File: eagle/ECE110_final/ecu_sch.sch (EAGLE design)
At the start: 1 part, among them IC1 MEGA8-AI

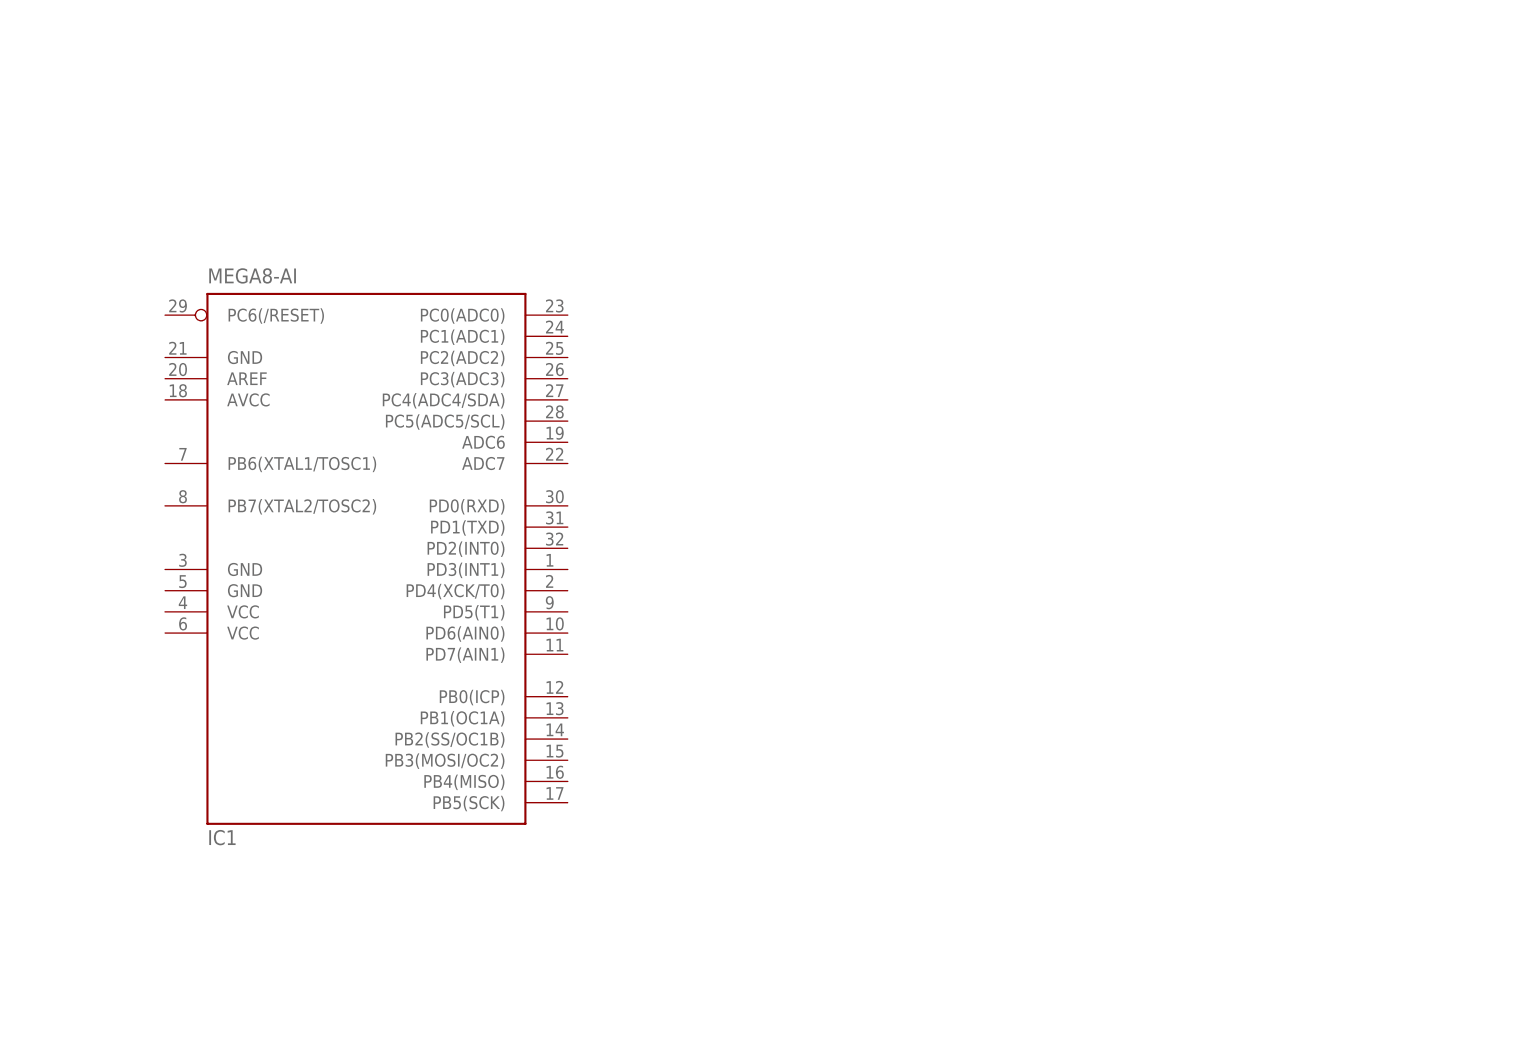
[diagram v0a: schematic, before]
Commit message: ECU Schematics: v1
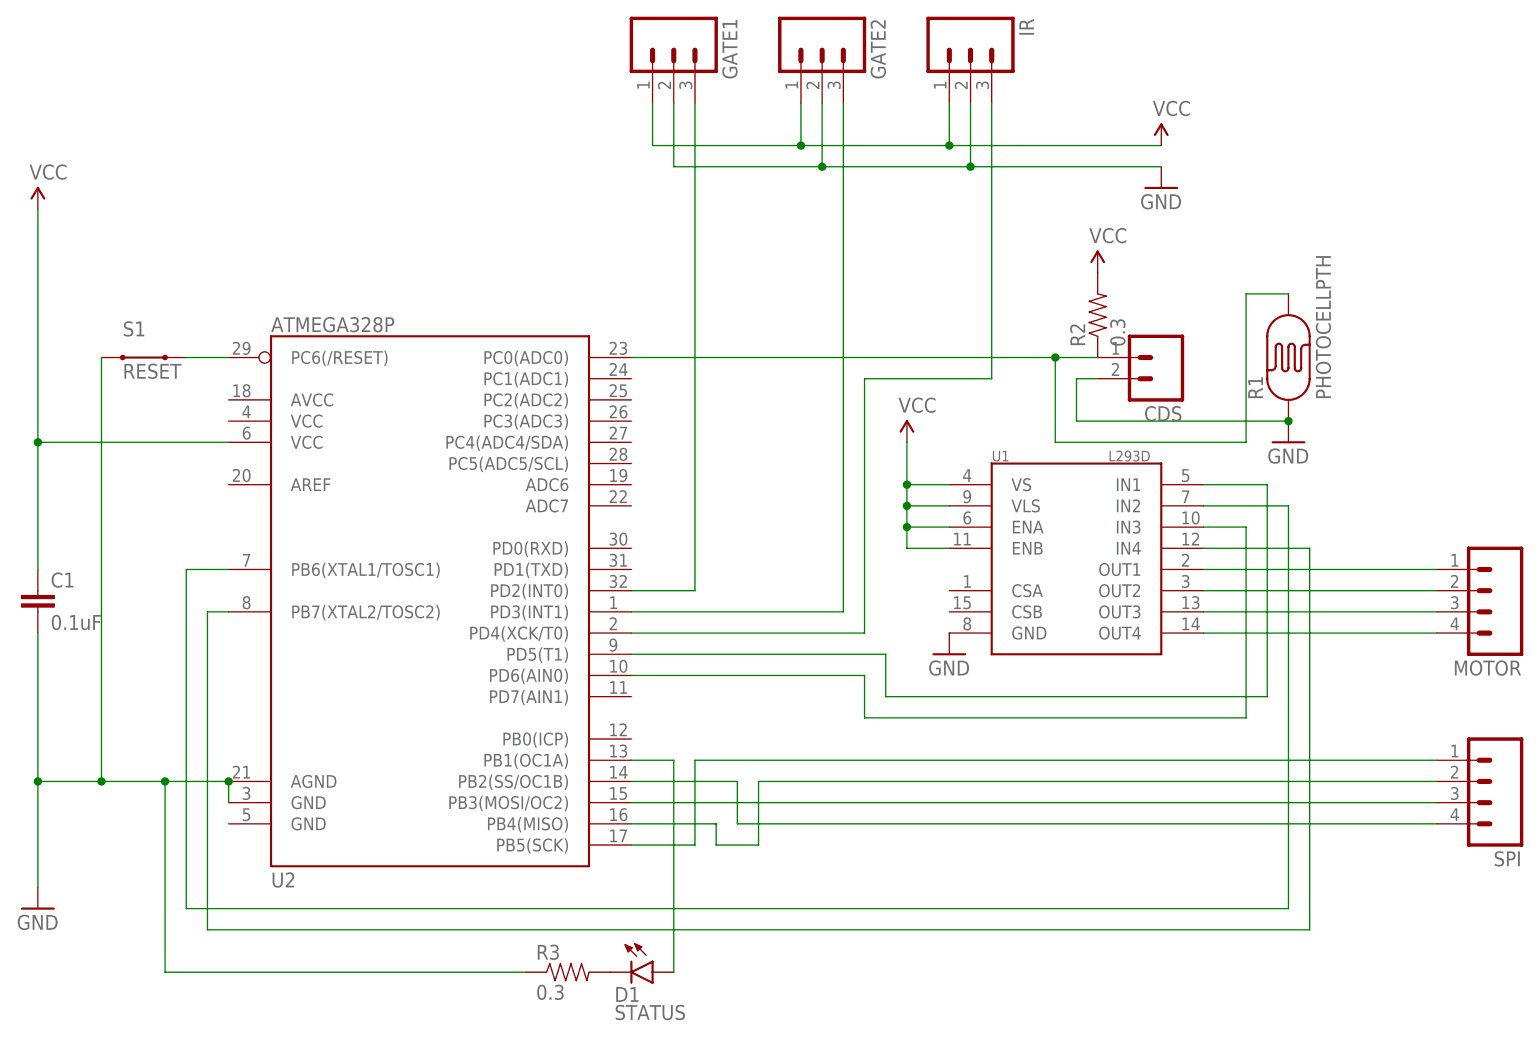
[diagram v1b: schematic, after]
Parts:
- removed IC1: MEGA8-AI, atmel:MEGA8-AI
- added C1: 0.1uF, SparkFun-Capacitors:0.1UF-25V(+80/-20%)(0603)
- added CDS: M02JST-PTH-2, SparkFun-Connectors:M02JST-PTH-2
- added D1: STATUS, SparkFun-LED:LED-WHITE
- added GATE1, GATE2, IR: (no value), SparkFun-Connectors:M03JST-PTH
- added MOTOR, SPI: (no value), SparkFun-Connectors:M04JST-PTH
- added R1: PHOTOCELLPTH, SparkFun-Sensors:PHOTOCELLPTH
- added R2, R3: 0.3, SparkFun-Resistors:0.3OHM-1/8W-1%(0805)
- added S1: RESET, SparkFun-Electromechanical:SWITCH-MOMENTARY-2-CLOSED
- added U1: L293D, SparkFun-PowerIC:L298
- added U2: ATMEGA328P, SparkFun-DigitalIC:ATMEGA328_SMT
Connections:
- new net GND: C1.2, CDS.2, GATE1.2, GATE2.2, IR.2, R1.P$1, R3.1, S1.1, U1.GND, U2.AGND, U2.GND@1
- new net N$1: U1.IN1, U2.PD5(T1)
- new net N$10: SPI.3, U2.PB3(MOSI/OC2)
- new net N$11: SPI.2, U2.PB4(MISO)
- new net N$12: SPI.1, U2.PB5(SCK)
- new net N$13: GATE1.3, U2.PD2(INT0)
- new net N$14: GATE2.3, U2.PD3(INT1)
- new net N$15: IR.3, U2.PD4(XCK/T0)
- new net N$16: CDS.1, R1.P$2, R2.1, U2.PC0(ADC0)
- new net N$17: S1.2, U2.PC6(/RESET)
- new net N$18: D1.C, R3.2
- new net N$19: D1.A, U2.PB1(OC1A)
- new net N$2: U1.IN3, U2.PD6(AIN0)
- new net N$3: U1.IN2, U2.PB6(XTAL1/TOSC1)
- new net N$4: U1.IN4, U2.PB7(XTAL2/TOSC2)
- new net N$5: MOTOR.1, U1.OUT1
- new net N$6: MOTOR.2, U1.OUT2
- new net N$7: MOTOR.3, U1.OUT3
- new net N$8: MOTOR.4, U1.OUT4
- new net N$9: SPI.4, U2.PB2(SS/OC1B)
- new net VCC: C1.1, GATE1.1, GATE2.1, IR.1, R2.2, U1.ENA, U1.ENB, U1.VLS, U1.VS, U2.VCC@2
